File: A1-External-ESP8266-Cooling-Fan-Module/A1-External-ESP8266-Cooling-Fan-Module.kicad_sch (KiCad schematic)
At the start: 49 parts, among them J1 USB_B_Micro, J2 Fan connector, J4 PIR sensor, J7 Leds connector, Q1 SI2300, Q3 SI2301, Q4 SI2301, U1 ESP12-F, U1 LM2596S-ADJ, U2 SRV05-4, U3 AMS1117-3.3, U3 CH340C, U6 AM2320

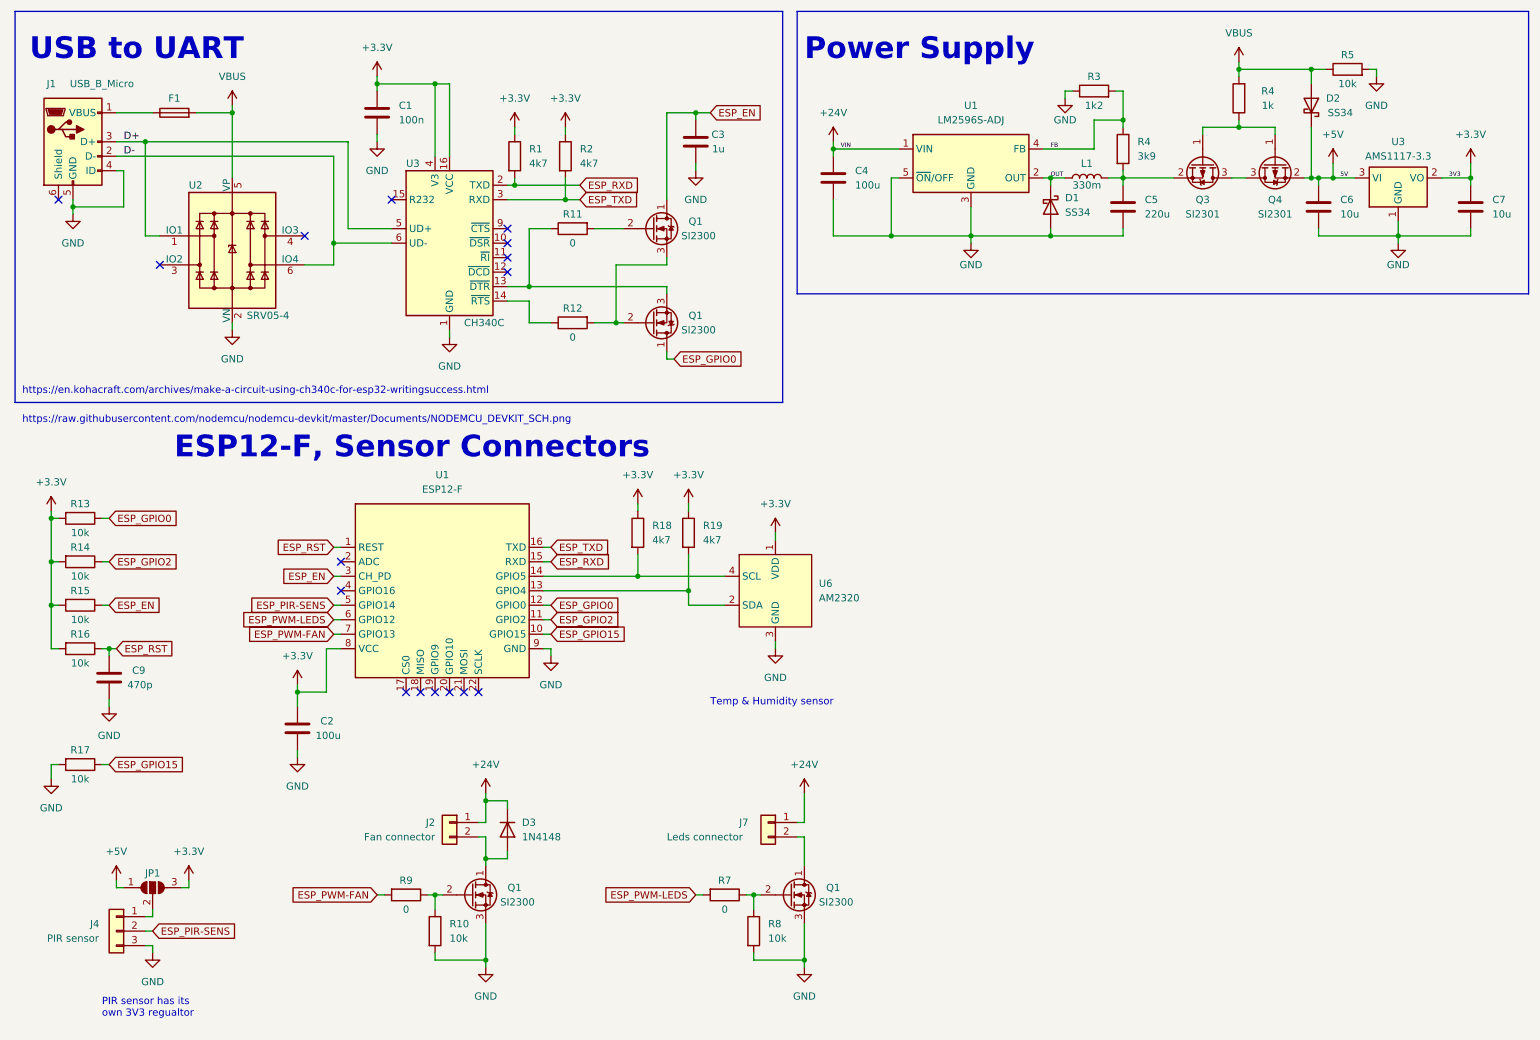
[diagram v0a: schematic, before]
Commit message: final layout
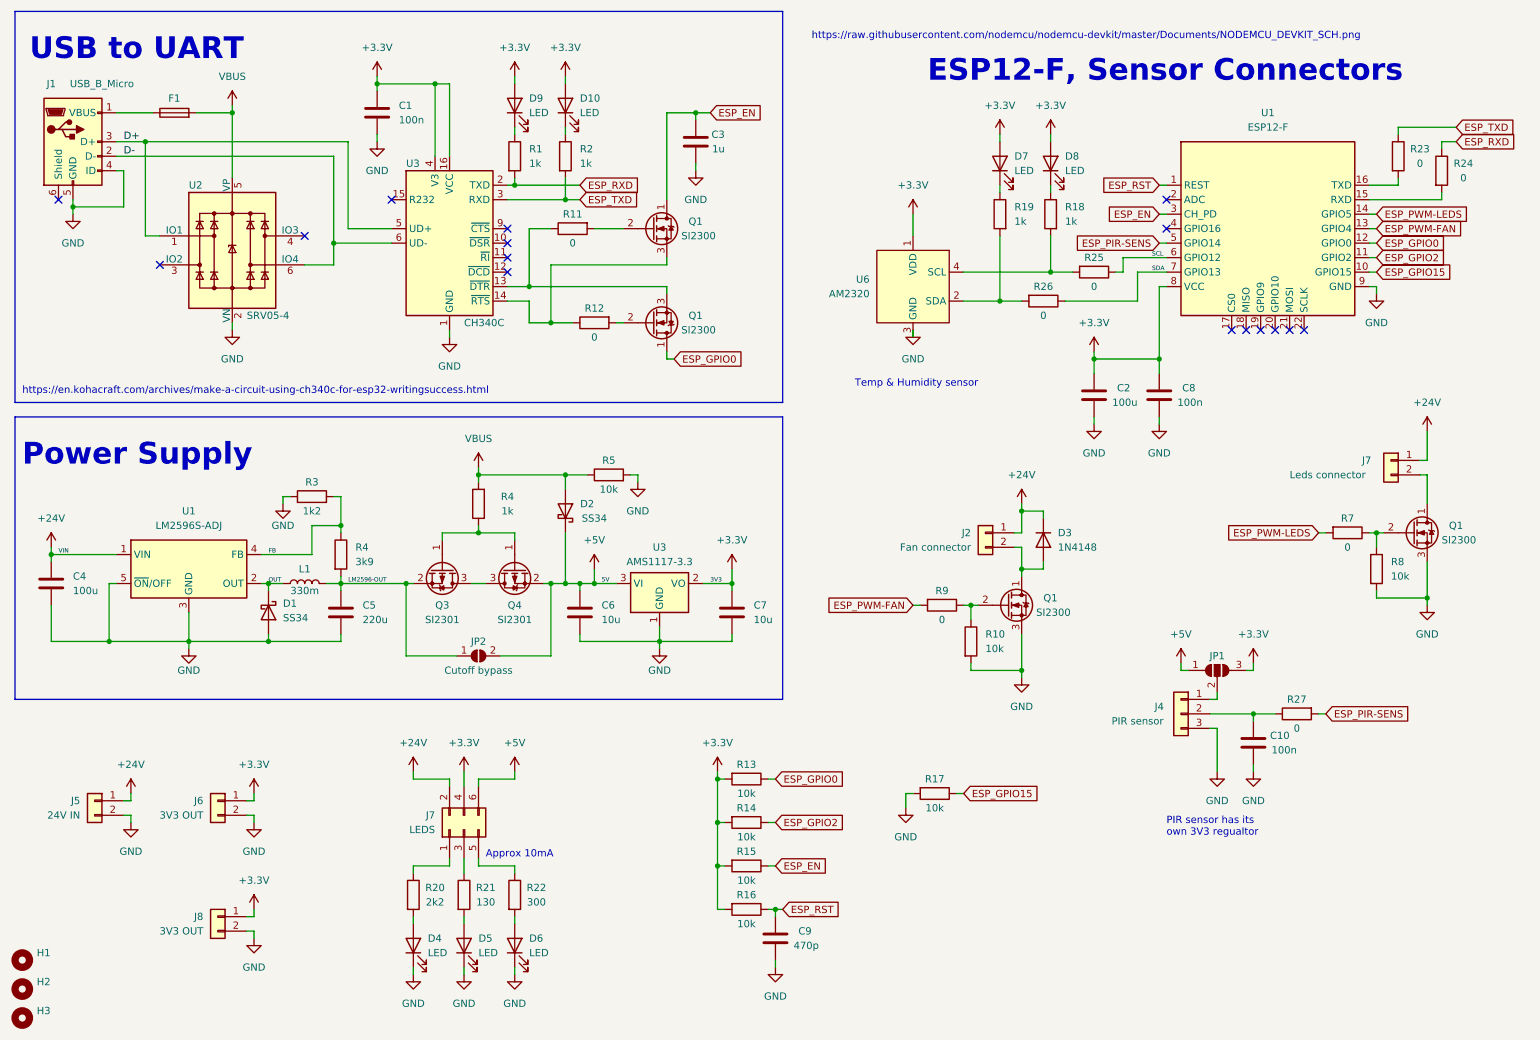
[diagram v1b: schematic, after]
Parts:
- added C10, C8: 100n, Capacitor_SMD:C_0603_1608Metric, symbol Device:C
- added D10, D4, D5, D6, D7, D8, D9: LED, LED_SMD:LED_0805_2012Metric, symbol Device:LED
- added H1, H2, H3: MountingHole, MountingHole:MountingHole_3.2mm_M3_DIN965_Pad, symbol Mechanical:MountingHole
- added J5: 24V IN, Connector_JST:JST_PH_B2B-PH-K_1x02_P2.00mm_Vertical, symbol Connector_Generic:Conn_01x02
- added J6, J8: 3V3 OUT, Connector_JST:JST_PH_B2B-PH-K_1x02_P2.00mm_Vertical, symbol Connector_Generic:Conn_01x02
- added J7: LEDS, Connector_PinHeader_2.54mm:PinHeader_2x03_P2.54mm_Vertical, symbol Connector_Generic:Conn_02x03_Odd_Even
- added JP2: Cutoff bypass, Jumper:SolderJumper-2_P1.3mm_Open_RoundedPad1.0x1.5mm, symbol Jumper:SolderJumper_2_Open
- added R20: 2k2, Resistor_SMD:R_0603_1608Metric, symbol Device:R
- added R21: 130, Resistor_SMD:R_0603_1608Metric, symbol Device:R
- added R22: 300, Resistor_SMD:R_0603_1608Metric, symbol Device:R
- added R23, R24, R25, R26, R27: 0, Resistor_SMD:R_0603_1608Metric, symbol Device:R
- C2: footprint Capacitor_SMD:C_1206_3216Metric -> Capacitor_SMD:CP_Elec_6.3x7.7
- C4: footprint Capacitor_THT:CP_Radial_D8.0mm_P3.80mm -> Capacitor_SMD:CP_Elec_8x10.5
- C5: footprint Capacitor_SMD:CP_Elec_6.3x7.7 -> Capacitor_SMD:CP_Elec_10x10.5
- J4: footprint (none) -> Connector_JST:JST_PH_B3B-PH-K_1x03_P2.00mm_Vertical
- R1, R18, R19, R2: value 4k7 -> 1k
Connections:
- net +24V: now also J5.1 (Pin_1), J7.2 (Pin_2)
- net +3.3V: now also C8.1, D10.2 (A), D7.2 (A), D8.2 (A), D9.2 (A), J6.1 (Pin_1), J7.4 (Pin_4), J8.1 (Pin_1); no longer R1.1, R18.1, R19.1, R2.1
- net +5V: now also J7.6 (Pin_6), JP2.2 (B)
- net ESP_PIR-SENS: now also R27.2; no longer J4.2 (Pin_2)
- net ESP_PWM-FAN: now also U1.13 (GPIO4); no longer U1.7 (GPIO13)
- net ESP_PWM-LEDS: now also U1.14 (GPIO5); no longer U1.6 (GPIO12)
- net ESP_RXD: now also R24.1; no longer U1.15 (RXD)
- net ESP_TXD: now also R23.1; no longer U1.16 (TXD)
- net GND: now also C10.2, C8.2, D4.1 (K), D5.1 (K), D6.1 (K), J5.2 (Pin_2), J6.2 (Pin_2), J8.2 (Pin_2)
- net at Q1.2 (G), R12.2: no longer Q1.3 (S)
- net LM2596-OUT: now reaches C5.1, L1.2, Q3.2 (S), R4.2
- net LM2596-OUT: now also JP2.1 (A)
- net at R12.1, U3.14 (~{RTS}): now also Q1.3 (S)
- net at R19.2, U6.2 (SDA): now also R26.2; no longer U1.13 (GPIO4)
- net at R18.2, U6.4 (SCL): now also R25.2; no longer U1.14 (GPIO5)
- new net: J7.3 (Pin_3), R21.1
- new net: D5.2 (A), R21.2
- new net: J7.5 (Pin_5), R22.1
- new net: D6.2 (A), R22.2
- new net: D7.1 (K), R19.1
- new net: D9.1 (K), R1.1
- new net: R24.2, U1.15 (RXD)
- new net: R23.2, U1.16 (TXD)
- new net: D8.1 (K), R18.1
- new net: J7.1 (Pin_1), R20.1
- new net: D10.1 (K), R2.1
- new net: C10.1, J4.2 (Pin_2), R27.1
- new net: D4.2 (A), R20.2
- new net SCL: R25.1, U1.6 (GPIO12)
- new net SDA: R26.1, U1.7 (GPIO13)
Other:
- note added: "Approx 10mA"
- moved on the sheet: C4, C5, C6, C7, C9, D1, D2, D3, J2, J4, J7, JP1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
